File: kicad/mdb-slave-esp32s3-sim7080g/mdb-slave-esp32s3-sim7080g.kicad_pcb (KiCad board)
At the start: 2 copper layers, 58.4 x 41 mm, 68 parts, among them J1 USB_C_Receptacle_USB2.0_16P, J2 JAE_SIM_Card_SF72S006, J3 Conn_02x11_Odd_Even, J4 Conn_Coaxial, J5 Conn_Coaxial, J6 MDB_Connector, Q1 NPN, Q2 NPN, Q3 NPN, SW1 SW_Push, U1 ESP32-S3FH4R2, U2 SIM7080G, U3 LM2594HVM-3.3, U4 TLP785, U5 TLP785, Y1 Crystal_GND24

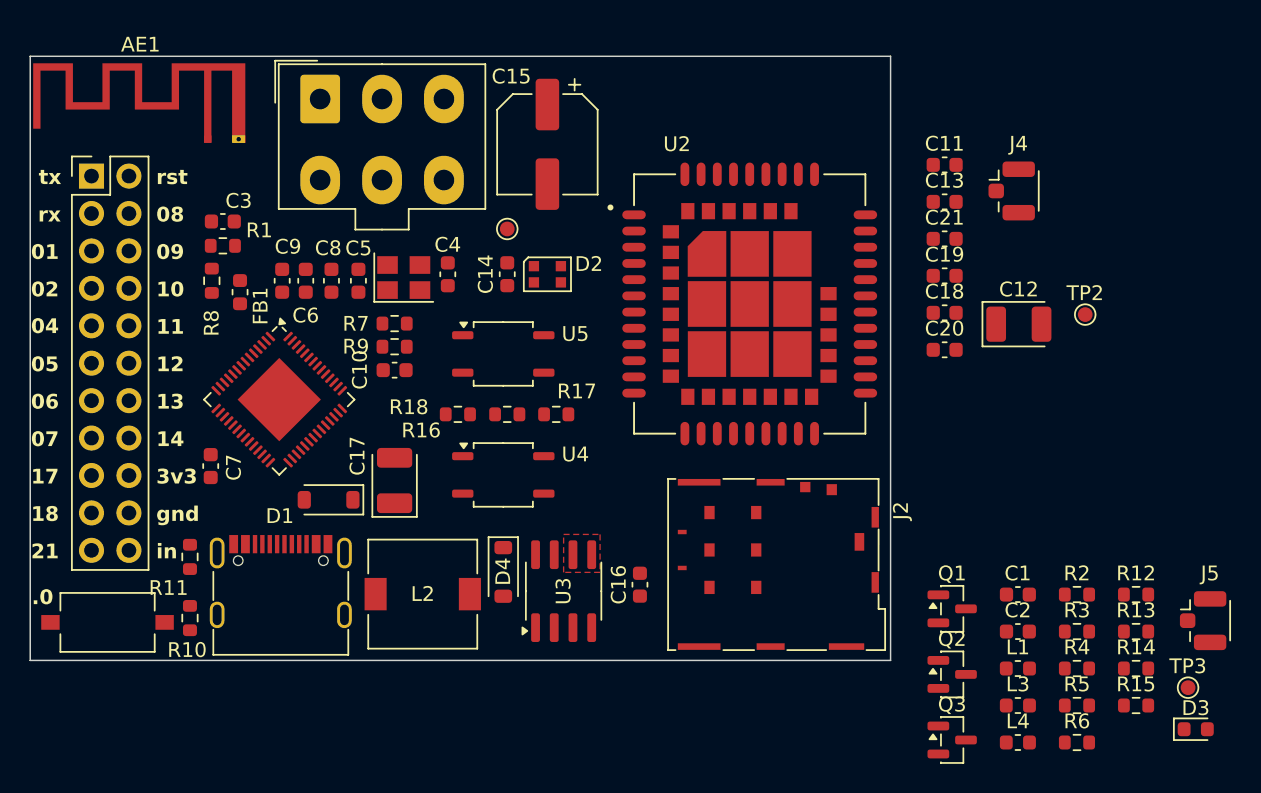
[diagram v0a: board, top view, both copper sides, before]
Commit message: Initial organization
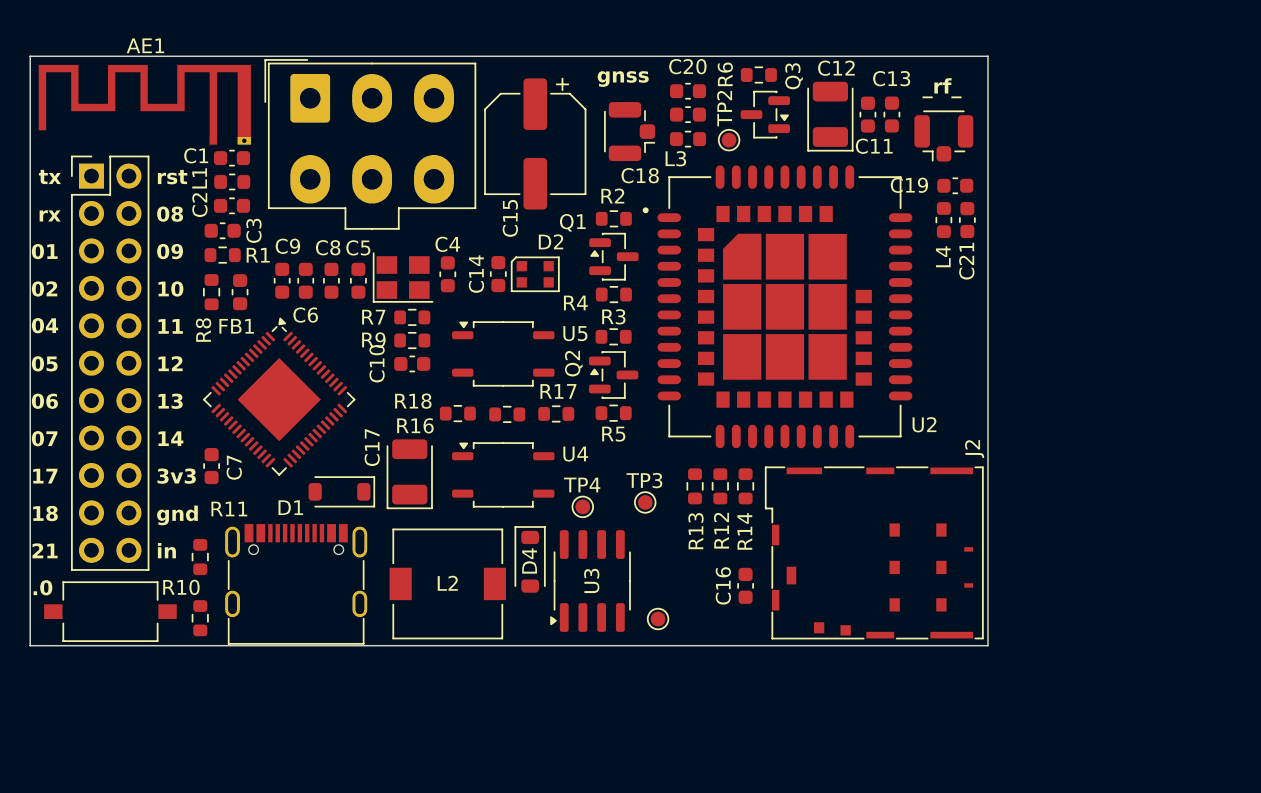
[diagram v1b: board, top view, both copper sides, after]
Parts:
- removed D3: LED, LED_SMD:LED_0603_1608Metric
- removed R15: 1k, Resistor_SMD:R_0603_1608Metric
- added TP4: TestPoint, TestPoint:TestPoint_Pad_D1.0mm, F.Cu at (206.0, 113.7)
- moved L1 62.7 mm to (182.2, 91.6)
- moved C1 61.0 mm to (182.2, 90.0), turned to 180 degrees
- moved C2 60.7 mm to (182.2, 93.2)
- moved R6 50.2 mm to (218.0, 84.4), turned to 180 degrees
- moved L3 44.5 mm to (213.1, 88.7)
- moved Q3 44.3 mm to (218.4, 87.0), turned to 180 degrees
- moved R2 40.5 mm to (208.1, 94.1)
- moved R4 40.4 mm to (208.1, 99.3)
- moved TP3 38.9 mm to (210.2, 113.4)
- moved R3 37.3 mm to (208.1, 102.1), turned to 180 degrees
- moved R5 37.2 mm to (208.1, 107.3)
- moved J5 37.2 mm to (230.5, 88.7), turned to 90 degrees
- moved L4 35.8 mm to (230.5, 94.2), turned to -90 degrees
- moved Q1 33.1 mm to (208.1, 96.7)
- moved R13 31.5 mm to (213.6, 112.3), turned to -90 degrees
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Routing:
- removed copper zone on F.Cu, net GND
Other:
- board size 58.4 x 41 mm -> 65 x 40 mm
- board text added: "_rf_"
- board text added: "gnss"
